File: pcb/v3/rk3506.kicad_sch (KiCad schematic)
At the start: 17 parts, among them J1 TestPoint, J15 TestPoint, J2 Conn_01x03, J3 TestPoint, U1 SOM3562_18

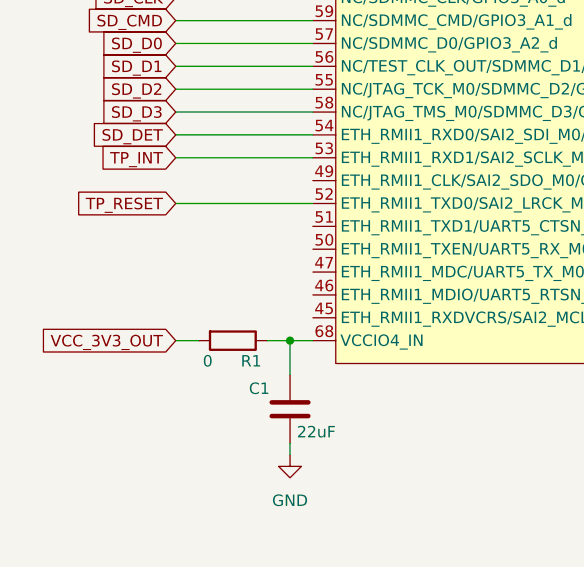
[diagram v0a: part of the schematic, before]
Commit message: pcb 3.9
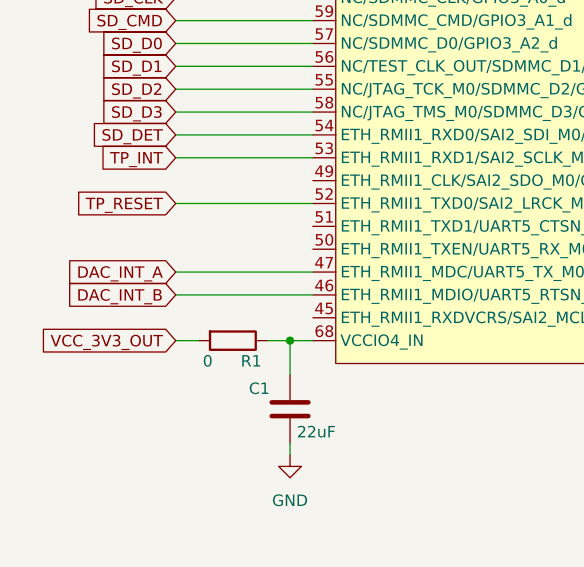
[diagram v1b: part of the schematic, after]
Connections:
- net DAC_INT_B: now reaches U1.46 (ETH_RMII1_MDIO/UART5_RTSN_M0/_GPIO3_B5_d)
- net DAC_INT_A: now reaches U1.47 (ETH_RMII1_MDC/UART5_TX_M0/GPIO3_B4_d)
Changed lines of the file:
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@@
+	(wire
+		(pts
+			(xy 68.58 194.31) (xy 83.82 194.31)
+		)
+		(stroke
+			(width 0)
+			(type default)
+		)
+	)
 	(wire
 		(pts
@@
 	(wire
 		(pts
+			(xy 68.58 191.77) (xy 83.82 191.77)
+		)
+		(stroke
+			(width 0)
+			(type default)
+		)
+	)
+	(wire
+		(pts
 			(xy 261.62 204.47) (xy 261.62 205.74)
 		)
@@
 		)
 	)
+	(global_label "DAC_INT_A"
+		(shape input)
+		(at 68.58 191.77 180)
+		(fields_autoplaced yes)
+		(effects
+			(font
+				(size 1.27 1.27)
+			)
+			(justify right)
+		)
+		(property "Intersheetrefs" "${INTERSHEET_REFS}"
+			(at 56.0395 191.77 0)
+			(effects
+				(font
+					(size 1.27 1.27)
+				)
+				(justify right)
+				(hide yes)
+			)
+		)
+	)
 	(global_label "VCC_1V8_OUT"
 		(shape input)
@@
 				(hide yes)
 			)
+		)
+	)
+	(global_label "DAC_INT_B"
+		(shape input)
+		(at 68.58 194.31 180)
+		(fields_autoplaced yes)
+		(effects
+			(font
+				(size 1.27 1.27)
+			)
+			(justify right)
+		)
+		(property "Intersheetrefs" "${INTERSHEET_REFS}"
+			(at 55.8581 194.31 0)
+			(effects
+				(font
+					(size 1.27 1.27)
+				)
+				(justify right)
+				(hide yes)
+			)
